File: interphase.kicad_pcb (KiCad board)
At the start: 2 copper layers, 139.7 x 141 mm, 115 parts, among them J1 Conn_01x04_Male, SW11 MOM-SPST, SW12 MOM-SPST, SW13 MOM-SPST, SW14 MOM-SPST, SW15 MOM-SPST, SW16 MOM-SPST, SW17 MOM-SPST, SW18 MOM-SPST, SW19 MOM-SPST, SW2 MOM-SPST, SW20 MOM-SPST, SW21 MOM-SPST, SW22 MOM-SPST, SW23 MOM-SPST, SW24 MOM-SPST, SW25 MOM-SPST, SW26 MOM-SPST, SW27 MOM-SPST, SW28 MOM-SPST, SW29 MOM-SPST, SW3 MOM-SPST, SW30 MOM-SPST, SW31 MOM-SPST, SW32 MOM-SPST, SW33 MOM-SPST, SW34 MOM-SPST, SW35 MOM-SPST, SW4 MOM-SPST, SW5 MOM-SPST, SW6 MOM-SPST, SW7 MOM-SPST, SW8 MOM-SPST, SW9 MOM-SPST, U1 Core51822B, U2 MCP1640, U3 MCP1640, U4 Core51822B

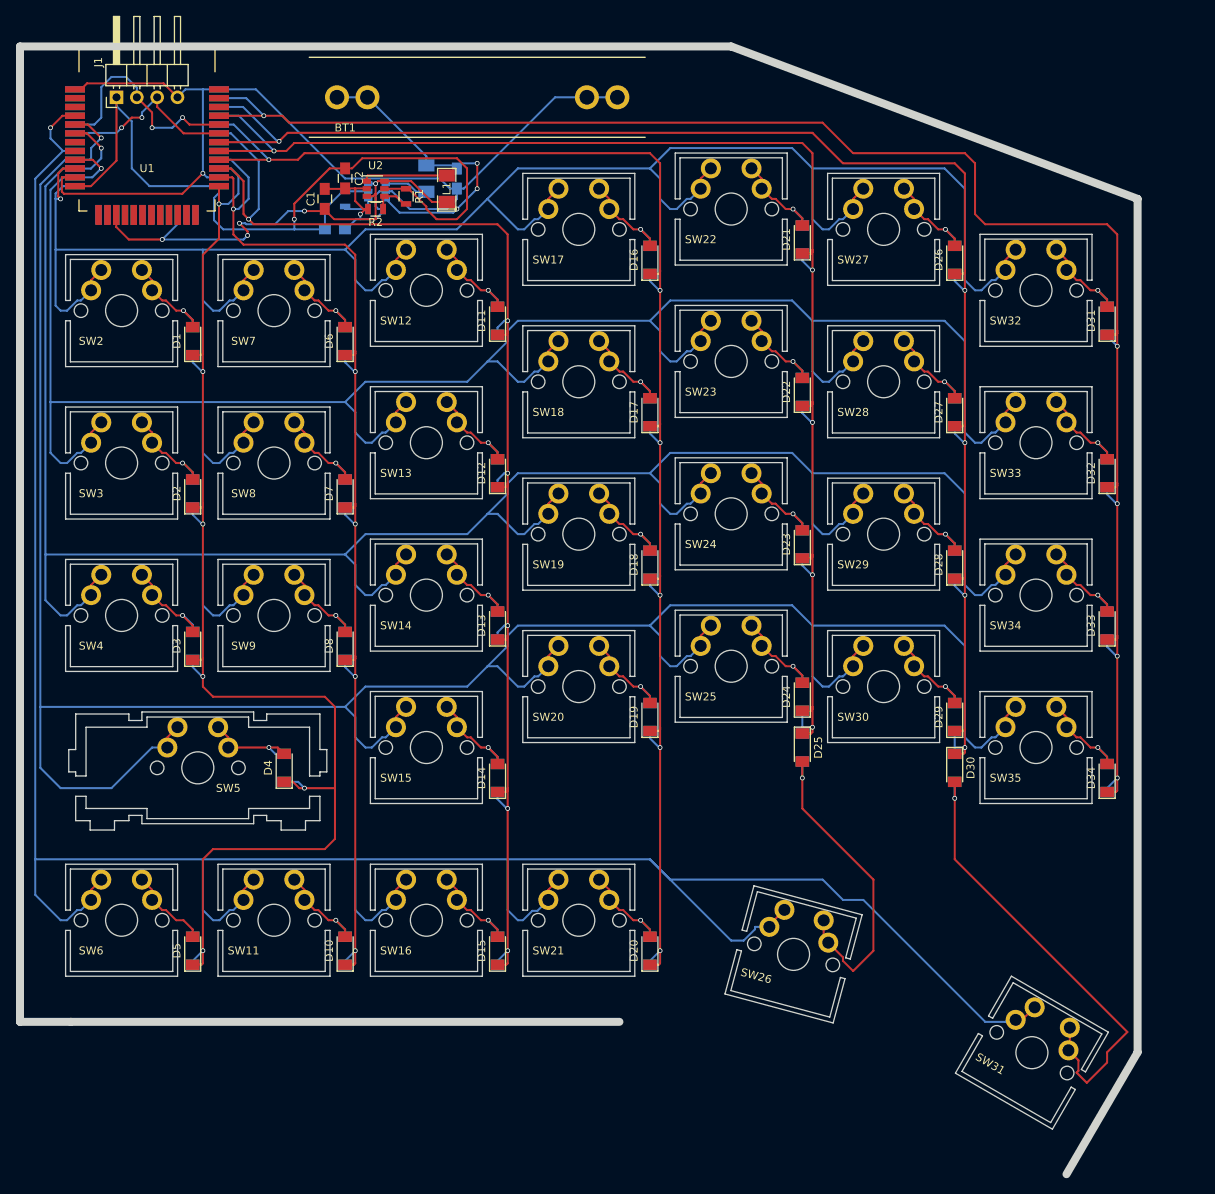
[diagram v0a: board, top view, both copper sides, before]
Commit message: re-routing
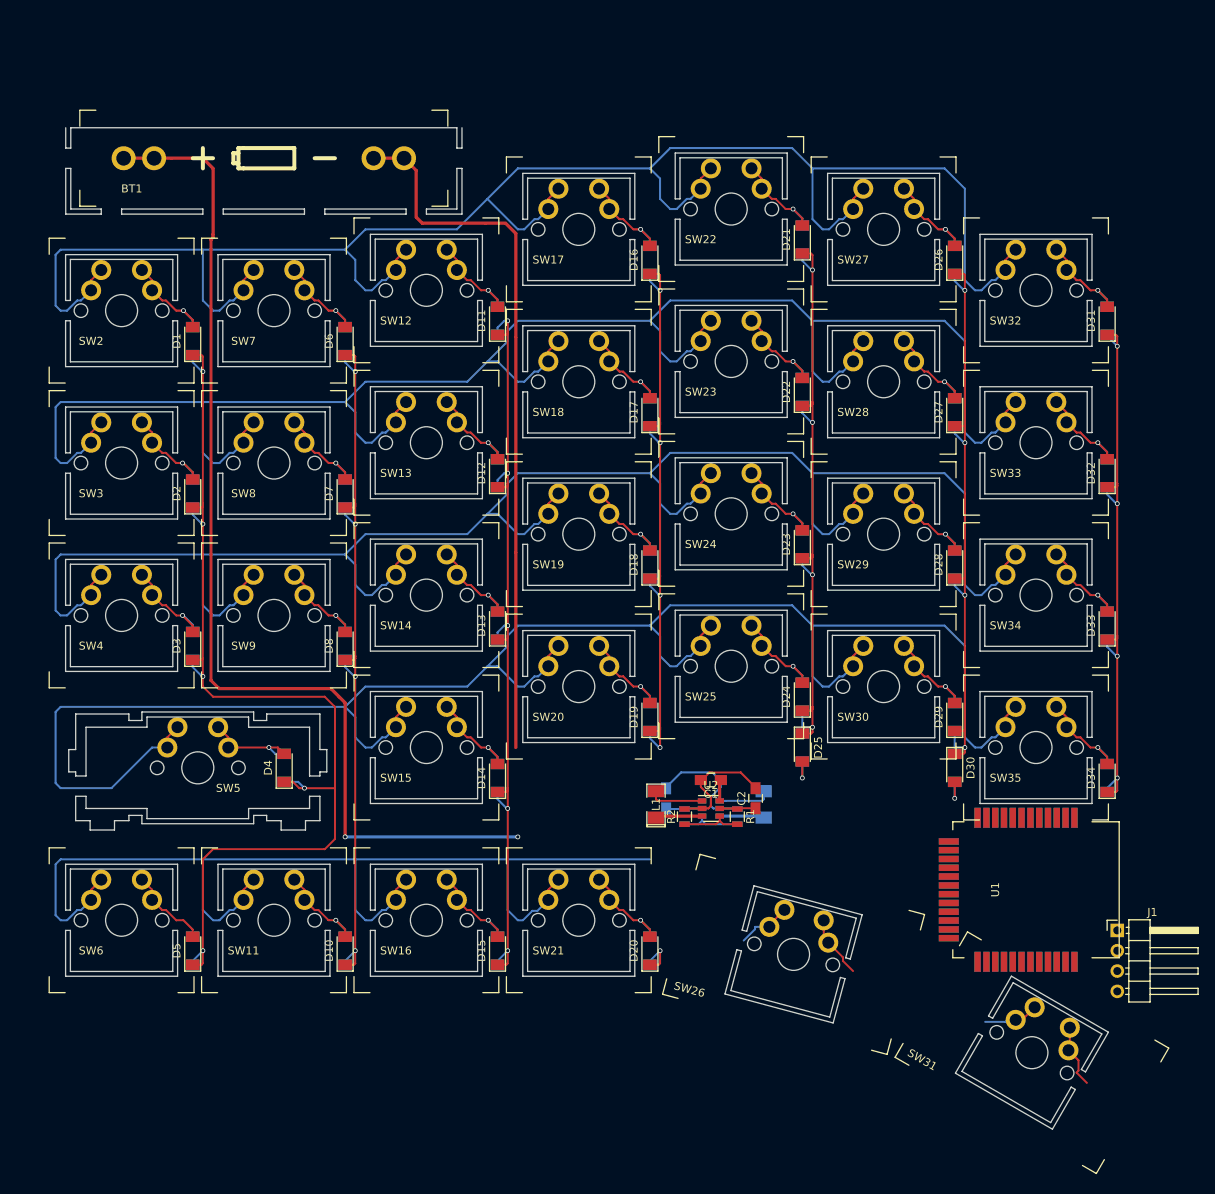
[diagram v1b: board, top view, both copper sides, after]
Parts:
- SW26, SW31: footprint Misc:CHERRY-MX_double_bo_nodiode -> Misc:CHERRY-MX_double_bo_1_5u
- moved J1 162.8 mm to (205.7, 124.5), turned to 0 degrees
- moved U1 146.4 mm to (195.6, 119.4), turned to 270 degrees
- moved U4 146.4 mm to (195.6, 119.4), turned to 90 degrees
- moved C2 92.9 mm to (160.5, 108.0), turned to 90 degrees
- moved L2 88.9 mm to (161.5, 108.7), turned to 90 degrees
- moved R7 88.4 mm to (158.2, 110.2), turned to 90 degrees
- moved R6 88.1 mm to (151.6, 110.2)
- moved U2 88.1 mm to (154.9, 109.2)
- moved R1 87.9 mm to (158.2, 110.2)
- moved U3 87.7 mm to (154.9, 109.2)
- moved C1 87.2 mm to (154.9, 105.7), turned to 180 degrees
- moved R2 85.2 mm to (151.6, 110.2), turned to 90 degrees
- moved C4 82.3 mm to (149.4, 108.0), turned to 90 degrees
- moved C3 81.6 mm to (154.9, 105.7), turned to 0 degrees
- moved L1 81.3 mm to (148.1, 108.7)
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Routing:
- net Net-(SW11-Pad1): track 320.8 -> 151.9 mm, vias 1 -> 0
- net Net-(D31-Pad1): track 214.0 -> 72.3 mm, vias 5 -> 4
- net Net-(D26-Pad1): track 197.2 -> 79.1 mm, vias 5 -> 4
- net Net-(D16-Pad1): track 184.9 -> 81.1 mm, vias 6 -> 5
- net +3V3: track 109.0 -> 9.22 mm, vias 1 -> 0
- net Net-(D21-Pad1): track 176.2 -> 79.4 mm, vias 5 -> 4
- net Net-(SW15-Pad1): track 311.6 -> 228.5 mm, vias 1 -> 0
- net Net-(D11-Pad1): track 167.7 -> 100.8 mm, vias 6 -> 5
- net Net-(SW14-Pad1): track 293.4 -> 231.4 mm, vias 1 -> 0
- net Net-(D10-Pad1): track 140.0 -> 92.1 mm, vias 5 -> 4
- net Net-(D30-Pad2): track 58.8 -> 12.2 mm
- net +BATT: track 100.3 -> 146.2 mm, vias 8 -> 2
- net Net-(SW13-Pad1): track 270.4 -> 231.4 mm, vias 1 -> 0
- net Net-(D1-Pad1): track 161.8 -> 131.3 mm, vias 6 -> 5
- net Net-(D25-Pad2): track 40.8 -> 12.0 mm
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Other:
- board size 139.7 x 141 mm -> 49.5 x 10.8 mm
- net class Bat added: clearance 0.2, trace_width 0.4, via_dia 0.6, via_drill 0.4
- net class nrf removed
